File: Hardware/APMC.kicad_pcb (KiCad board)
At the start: 2 copper layers, 85 x 52.5 mm, 148 parts, among them J1 Pin header Male 2x7 P:1.27, J10 Conn_01x03, J11 Conn_01x03, J12 Conn_01x08, J13 Conn_01x03, J14 Conn_01x04, J2 USB-C receptacle, J5 Terminal 1x5 P:3.5mm, J6 Terminal 1x5 P:3.5mm, J7 Terminal 1x5 P:3.5mm, J8 Conn_01x04, J9 Conn_01x04, M1 Logo_Open_Hardware_Small, Q1 DMP6023LE, Q2 DMP6023LE, Q3 DMP6023LE, Q4 BSS123, Q5 DMP6023LE, Q6 DMP6023LE, Q7 BSS123, Q8 DMP3056L, U1 LMR51610, U10 TXU0202, U11 PCA9306, U12 LM74703/LM74704, U13 TPS62162DSG, U2 LCFE201202A, U3 TXU0202, U4 M95P32, U5 STM32U575CITx, U6 XTR200, U7 TPS7A2031PDBVR, U8 XTR200, U9 ADS1x2S14, X1 SiT8008Bx-7x, Y1 32.768kHz

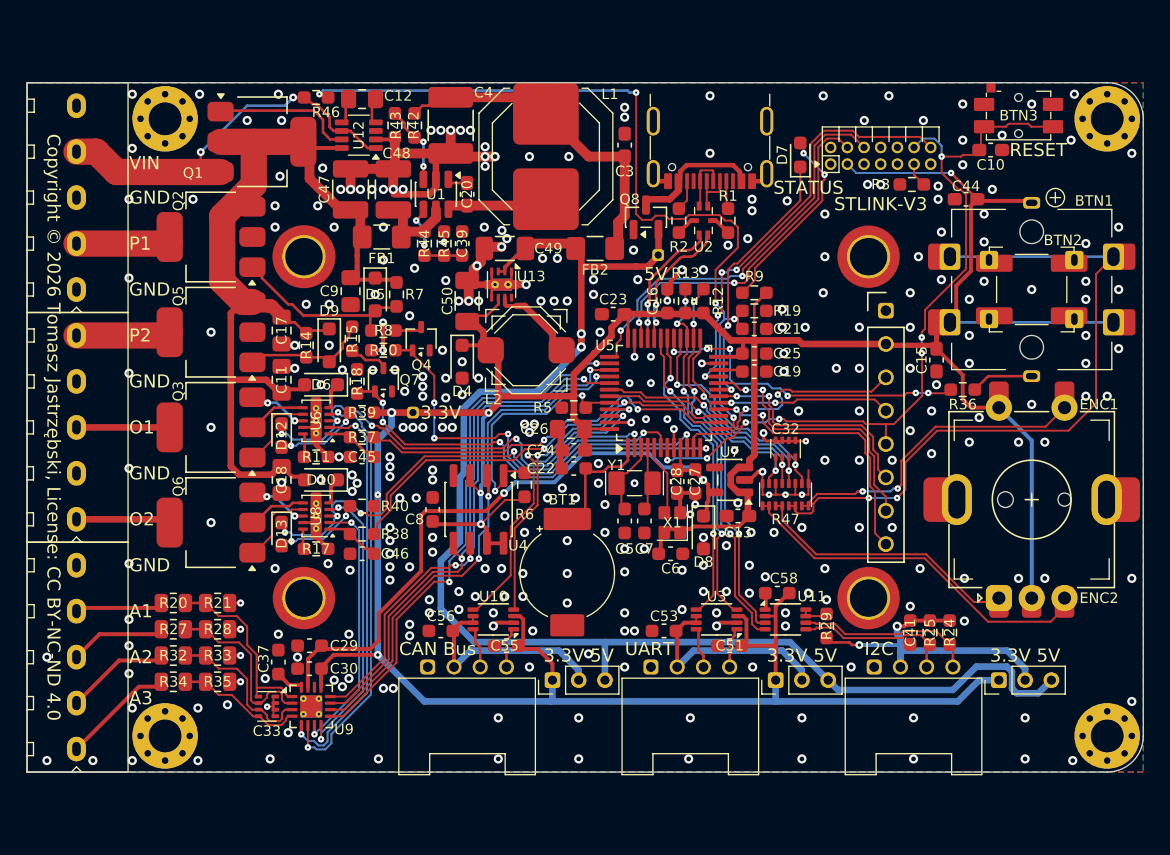
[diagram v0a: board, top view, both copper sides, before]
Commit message: PCB refined
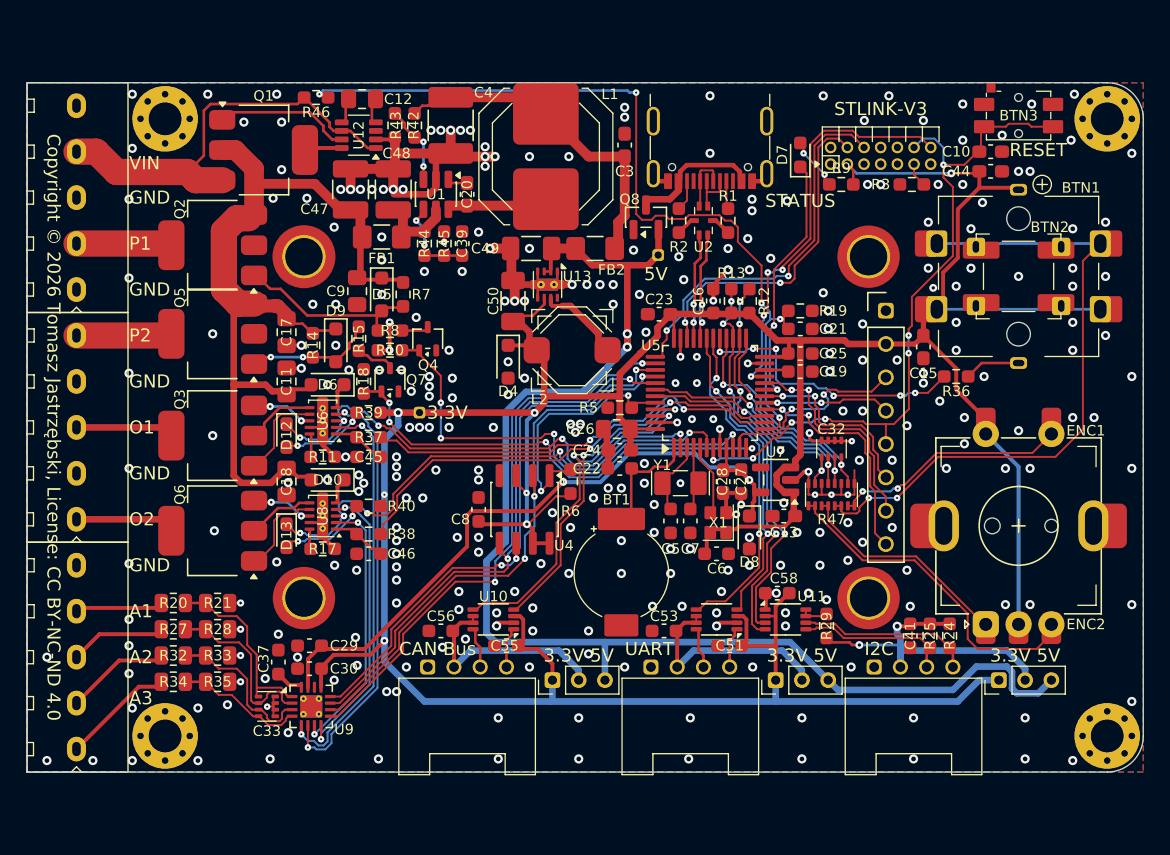
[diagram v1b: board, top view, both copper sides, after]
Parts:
- moved R9 10.6 mm to (89.5, 20.8)
- moved BT1 4.12 mm to (72.8, 50.4)
- moved R6 3.51 mm to (68.9, 43.4)
- moved C13 3.50 mm to (85.1, 46.0)
- moved C16 3.50 mm to (79.8, 29.6)
- moved C19 3.50 mm to (86.4, 35.0)
- moved C21 3.50 mm to (86.4, 31.8)
- moved C22 3.50 mm to (72.6, 42.4)
- moved C23 3.50 mm to (75.6, 30.6)
- moved C24 3.50 mm to (72.6, 41.0)
- moved C25 3.50 mm to (86.4, 33.6)
- moved C26 3.50 mm to (72.4, 39.4)
- moved C27 3.50 mm to (80.5, 43.4)
- moved C28 3.50 mm to (81.9, 43.4)
- moved C32 3.50 mm to (88.8, 40.9)
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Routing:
- net Net-(D7-A): track 14.9 -> 4.20 mm
- net /C: track 24.3 -> 17.8 mm
- net /5V: track 104.3 -> 99.5 mm
- net /NRST: track 58.4 -> 53.8 mm
- net /A: track 20.7 -> 16.8 mm
- net /D: track 53.1 -> 49.4 mm
- net /LCD_DC: track 17.5 -> 14.0 mm
- net /LCD_PWM: track 21.0 -> 17.5 mm
- net /LCD_MOSI: track 13.3 -> 9.82 mm
- net /LCD_CS: track 20.4 -> 16.9 mm
- net /LCD_SCK: track 18.9 -> 15.4 mm
- net /PWM0: track 24.9 -> 21.7 mm
- net /EF2: track 38.7 -> 41.7 mm
- net /PWM2: track 31.9 -> 34.9 mm
- net /PWM1: track 32.4 -> 35.4 mm
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
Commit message: rev 2.1 work in progress
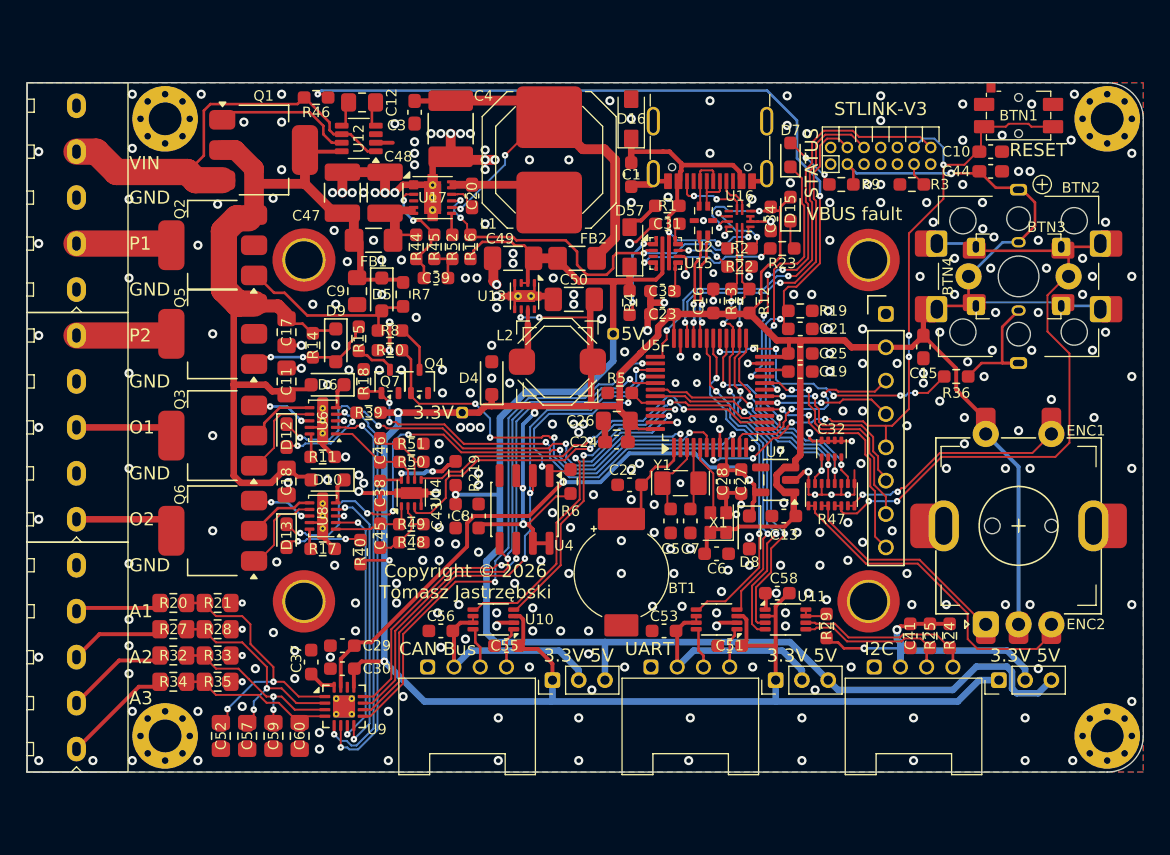
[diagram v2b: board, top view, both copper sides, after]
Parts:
- removed Q8: DMP3056L, Package_TO_SOT_SMD:SOT-23
- removed R37, R38: 10k, Resistor_SMD:R_0603_1608Metric_Pad0.98x0.95mm_HandSolder
- removed R42: 19.1k, Resistor_SMD:R_0603_1608Metric_Pad0.98x0.95mm_HandSolder
- removed R43: 100k, Resistor_SMD:R_0603_1608Metric_Pad0.98x0.95mm_HandSolder
- removed U1: LMR51610, Package_TO_SOT_SMD:SOT-23-6
- added BTN4: SW_Push, Custom:Schurter_MCS-18a, F.Cu at (103.0, 27.8)
- added C1: 1uF/10V, Custom:C_0603_1608Metric_Pad0.98x0.95mm_HandSolder, F.Cu at (73.5, 20.0)
- added C31: 1.5nF, Custom:C_0603_1608Metric_Pad0.98x0.95mm_HandSolder, F.Cu at (76.2, 23.8)
- added C34: 100nF, Custom:C_0603_1608Metric_Pad0.98x0.95mm_HandSolder, F.Cu at (84.1, 23.4)
- added C38: 1uF/10V, Custom:C_0603_1608Metric_Pad0.98x0.95mm_HandSolder, F.Cu at (54.4, 44.2)
- added C43: 1uF/10V, Custom:C_0603_1608Metric_Pad0.98x0.95mm_HandSolder, F.Cu at (60.1, 46.0)
- added C52: 100pF, Custom:0603_0805, F.Cu at (42.2, 62.8)
- added C57: 100pF, Custom:0603_0805, F.Cu at (44.2, 62.8)
- added C59: 100pF, Custom:0603_0805, F.Cu at (46.2, 62.8)
- added C60: 100pF, Custom:0603_0805, F.Cu at (48.2, 62.8)
- added D15: Red LED, Custom:LED_0603_1608Metric_Pad1.05x0.95mm_HandSolder, F.Cu at (85.6, 22.6)
- added D16: TVS 5V U, Custom:D_SOD-123F, F.Cu at (73.5, 15.8)
- added D57: SS10200HE, Custom:D_SOD-123F, F.Cu at (73.4, 25.5)
- added R16: 100k, Resistor_SMD:R_0603_1608Metric_Pad0.98x0.95mm_HandSolder, F.Cu at (61.2, 25.5)
- added R219: 330R/200mA, Resistor_SMD:R_0603_1608Metric_Pad0.98x0.95mm_HandSolder, F.Cu at (60.1, 42.8)
- added R22: 5.6k, Resistor_SMD:R_0603_1608Metric_Pad0.98x0.95mm_HandSolder, F.Cu at (81.8, 27.0)
- added R23: 680R, Resistor_SMD:R_0603_1608Metric_Pad0.98x0.95mm_HandSolder, F.Cu at (85.0, 25.6)
- added R4: 360k, Resistor_SMD:R_0603_1608Metric_Pad0.98x0.95mm_HandSolder, F.Cu at (73.4, 29.8)
- added R48: 162k, Resistor_SMD:R_0603_1608Metric_Pad0.98x0.95mm_HandSolder, F.Cu at (56.8, 48.0)
- added R49: 115k, Resistor_SMD:R_0603_1608Metric_Pad0.98x0.95mm_HandSolder, F.Cu at (56.8, 46.6)
- added R50: 115k, Resistor_SMD:R_0603_1608Metric_Pad0.98x0.95mm_HandSolder, F.Cu at (56.8, 41.9)
- added R51: 162k, Resistor_SMD:R_0603_1608Metric_Pad0.98x0.95mm_HandSolder, F.Cu at (56.8, 40.5)
- added R52: 64.9k, Resistor_SMD:R_0603_1608Metric_Pad0.98x0.95mm_HandSolder, F.Cu at (59.9, 25.5)
- added U14: OPA2387DSG, Custom:WSON-8-1EP_2x2mm_P0.5mm_EP0.9x1.6mm, F.Cu at (56.8, 44.2)
- added U15: TPS259461A, Custom:VQFN-HR-10-RPW, F.Cu at (76.1, 26.0)
- added U16: TUSB320, Package_DFN_QFN:Texas_X2QFN-12_1.6x1.6mm_P0.4mm, F.Cu at (81.8, 23.4)
- added U17: LMR38015, Custom:TI_WSON-12-1EP_3x3mm_P0.5mm_EP1.3x2.5mm_ThermalVias, F.Cu at (58.4, 21.8)
- BTN3: renamed from BTN2; footprint Custom:tactile_switch_6x6 -> Custom:tactile_switch_6x6_LED
- C13: value 1uF/4V -> 4.7uF/6.3; footprint Capacitor_SMD:C_0603_1608Metric_Pad1.08x0.95mm_HandSolder -> Custom:C_0603_1608Metric_Pad0.98x0.95mm_HandSolder
- C28: value 4.7uF/4V -> 1uF/10V
- C33: value 10nF -> 1.5nF; footprint Custom:RC_Array_Isolated_4_0805 -> Custom:C_0603_1608Metric_Pad0.98x0.95mm_HandSolder
- C45, C46: value 10nF -> 100pF
- J2: value USB-C receptacle -> USB4105-GF-A
- L1: value 33uH -> 22uH
- Q1: value DMP6023LE -> FDT86102LZ
- R1: value 5.1k -> 11R
- R11, R17: value 1k -> 1.69k
- R2: value 5.1k -> 887k
- R20, R21, R27, R28, R32, R33, R34, R35: footprint Resistor_SMD:R_0805_2012Metric -> Custom:0603_0805
- R45: value 25.5k -> 27k
- R5: value 10k -> 100k
- moved C33 43.7 mm to (75.9, 28.9)
- moved C3 16.2 mm to (57.0, 15.2), turned to 90 degrees
- moved C46 7.92 mm to (54.4, 41.0), turned to -90 degrees
- moved J4 6.91 mm to (72.1, 32.1)
- moved C45 6.06 mm to (54.4, 47.5), turned to 90 degrees
- moved R2 5.09 mm to (81.8, 25.6), turned to 0 degrees
- moved R1 4.76 mm to (76.2, 22.4), turned to 0 degrees
- moved C50 4.63 mm to (69.1, 29.5), turned to 180 degrees
- moved R40 3.56 mm to (52.9, 48.8), turned to 90 degrees
- moved Q4 3.31 mm to (57.4, 35.8)
- moved C39 3.30 mm to (58.6, 27.9), turned to 180 degrees
- moved J3 3.25 mm to (60.6, 38.1)
- moved C29 2.50 mm to (51.5, 55.9)
- moved C30 2.50 mm to (51.5, 57.6)
- moved C37 2.50 mm to (49.1, 57.1)
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- renumbered BTN3 to BTN1, BTN1 to BTN2
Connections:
- BTN2 pad 3: Net-(BTN1-K) -> Net-(BTN2-K)
- C13 pad 1: /VDD -> GND
- C13 pad 2: GND -> /VDD
- C33 pad 1: /ADC1 -> GND
- C33 pad 2: /ADC2 -> Net-(U15-DVDT)
- C45 pad 1: GND -> Net-(U14A--)
- C45 pad 2: Net-(U6-Input) -> Net-(U8-Input)
- C46 pad 1: GND -> Net-(U14B--)
- C46 pad 2: Net-(U8-Input) -> Net-(U6-Input)
- ENC2 pad B: /B -> unconnected-(ENC2-PadB)
- J2 pad A8: unconnected-(J2-SBU1-PadA8) -> (no net)
- J2 pad B8: unconnected-(J2-SBU2-PadB8) -> (no net)
- R1 pad 1: GND -> Net-(D57-A)
- R1 pad 2: /CC1 -> /USB_VBUS
- R2 pad 1: GND -> /USB_VBUS
- R2 pad 2: /CC2 -> Net-(U16-VBUS_DET)
- R36 pad 1: Net-(BTN1-K) -> Net-(BTN2-K)
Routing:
- net /PG5: track 0.00 -> 30.2 mm, vias 0 -> 4
- net /VDD: track 275.7 -> 296.3 mm, vias 7 -> 11
- net /USB_VBUS: track 9.52 -> 22.0 mm, vias 0 -> 2
- net Net-(U15-~{FLT}): track 0.00 -> 11.1 mm, vias 0 -> 2
- net /5V: track 99.5 -> 110.2 mm, vias 2 -> 1
- net Net-(BTN2-K): track 0.00 -> 10.0 mm
- net Net-(U17-FB): track 23.8 -> 33.0 mm, vias 0 -> 2
- net Net-(U14C-V+): track 0.00 -> 6.42 mm, vias 0 -> 2
- net /ADC1: track 13.7 -> 20.1 mm, vias 0 -> 2
- net Net-(U15-EN/UVLO): track 0.00 -> 6.26 mm, vias 0 -> 2
- net Net-(U1-FB): track 5.67 -> 0.00 mm, vias 2 -> 0
- net Net-(U16-VBUS_DET): track 0.00 -> 5.61 mm, vias 0 -> 2
- net Net-(U14A--): track 0.00 -> 5.56 mm
- net Net-(U14B--): track 0.00 -> 5.53 mm
- net /I2C_SCL: track 29.1 -> 33.9 mm
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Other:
- board text added: "All-purpose Micro Controller (APMC) rev. 2.1 2026-08-02"
- board text added: "Copyright © 2026 Tomasz Jastrzębski"
- board text removed: "All-purpose Micro Controller (APMC) rev. 2.0.1 2026-07-21"

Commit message: refinement
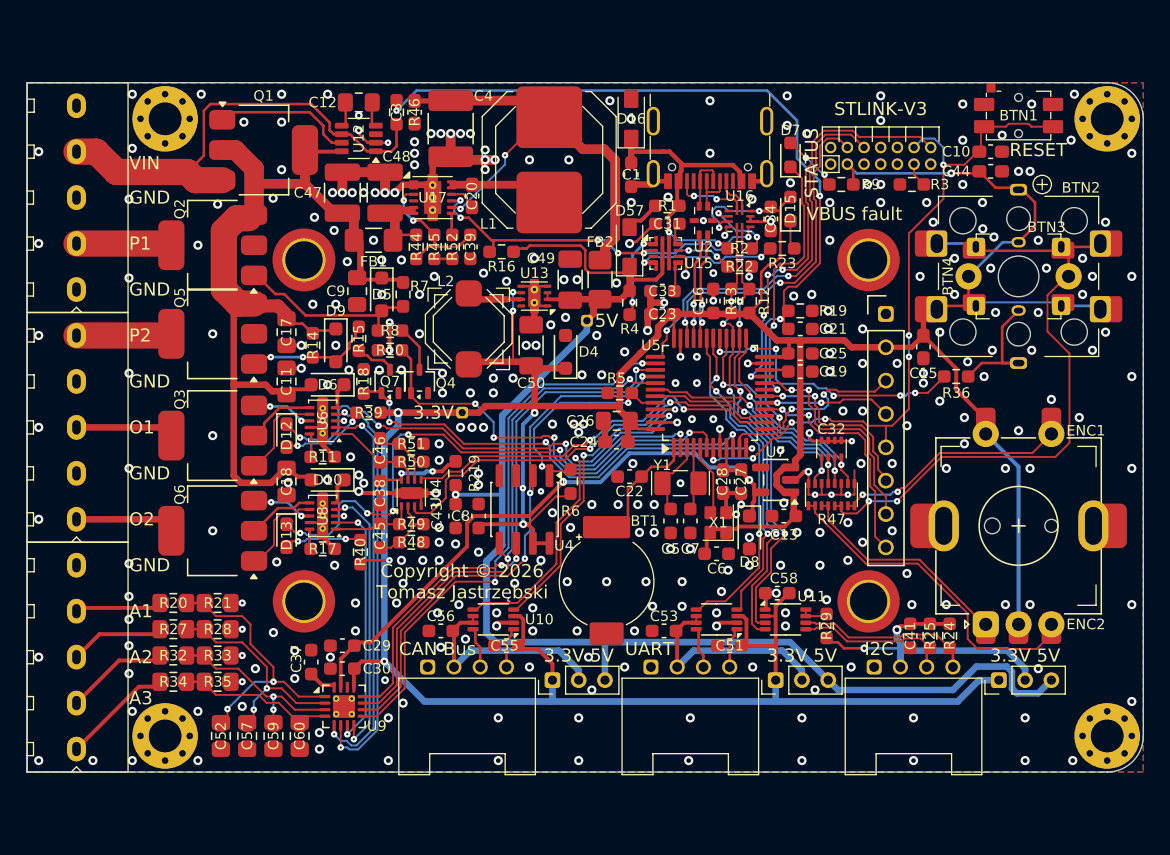
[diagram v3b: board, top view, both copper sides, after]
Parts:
- moved L2 7.20 mm to (61.1, 31.8), turned to -90 degrees
- moved R46 6.23 mm to (55.6, 15.2), turned to 90 degrees
- moved D4 5.97 mm to (68.5, 33.5)
- moved C50 4.78 mm to (65.9, 33.0), turned to 90 degrees
- moved C49 4.64 mm to (68.8, 28.0), turned to 90 degrees
- moved C39 3.54 mm to (61.2, 25.5), turned to 90 degrees
- moved R16 2.40 mm to (63.6, 25.9), turned to 180 degrees
- moved FB2 2.39 mm to (71.1, 28.0), turned to 90 degrees
- moved J4 2.24 mm to (70.1, 31.1)
- moved BT1 1.29 mm to (71.6, 51.0)
- moved U13 0.75 mm to (66.1, 29.2), turned to 180 degrees
- moved C22 0.62 mm to (73.4, 43.0)
- moved C12 0.25 mm to (52.8, 14.5)
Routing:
- net /ADC0: track 67.4 -> 61.9 mm
- net GND: track 94.0 -> 90.7 mm, vias 321 -> 333
- net /VIN: track 32.7 -> 35.7 mm
- net /5V: track 110.2 -> 107.7 mm
- net /VDD: track 296.3 -> 298.3 mm
- net /VBAT: track 5.73 -> 7.66 mm
- net Net-(U17-EN): track 8.47 -> 10.3 mm
- net /PG5: track 30.2 -> 28.6 mm, vias 4 -> 6
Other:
- board text added: "All-purpose Micro Controller (APMC) rev. 2.1 2026-08-22"
- board text removed: "All-purpose Micro Controller (APMC) rev. 2.1 2026-08-02"

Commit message: refinement
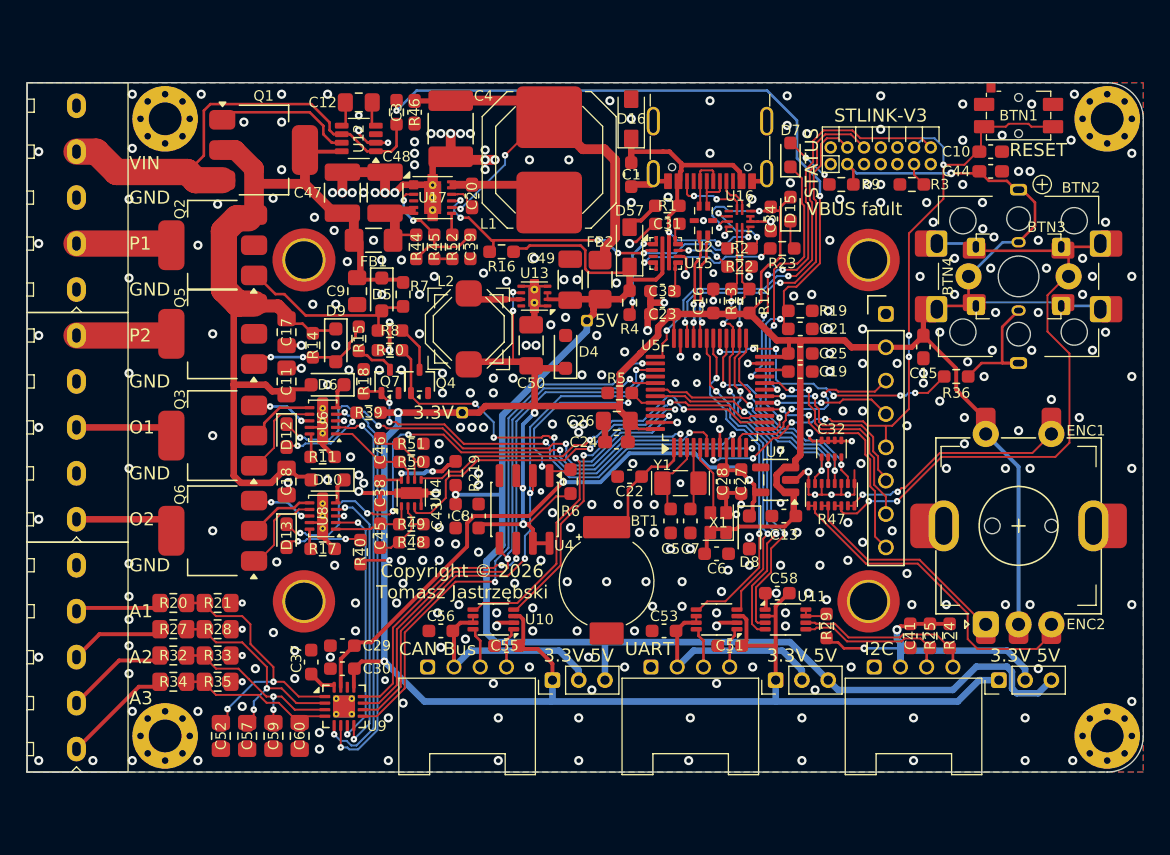
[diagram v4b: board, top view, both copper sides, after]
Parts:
- H1, H2, H3, H4: value M2.5x7 -> M2.5x6
- H10, H11, H12, H13: value Standoff_M2x4.0 -> Standoff_M2x3.0
- J1: footprint Custom:PinHeader_2x07_P1.27mm_Horizontal-UP -> Custom:PinHeader_2x07_P1.27mm_Horizontal-UP-0.15
- moved M1 4.44 mm to (52.1, 61.0)
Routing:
- net /VDD: track 298.3 -> 297.4 mm
- net GND: vias 333 -> 335
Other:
- board text added: "All-purpose Micro Controller (APMC) rev. 2.1 2026-08-23"
- board text removed: "All-purpose Micro Controller (APMC) rev. 2.1 2026-08-22"
